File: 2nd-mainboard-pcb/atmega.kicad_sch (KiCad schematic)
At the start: 23 parts, among them J17 Fan_12/5V_Regelung, J2 Fan_12/5V_Regelung, J3 FAN0, J4 FAN1, J5 FAN2, J6 FAN3, U10 ATmega328PB-A, U7 TPM16050-S6TR, U8 RJK0456DPB-00-J5, U9 RJK0456DPB-00-J5, Y1 ECS-160-18-4X-CKM

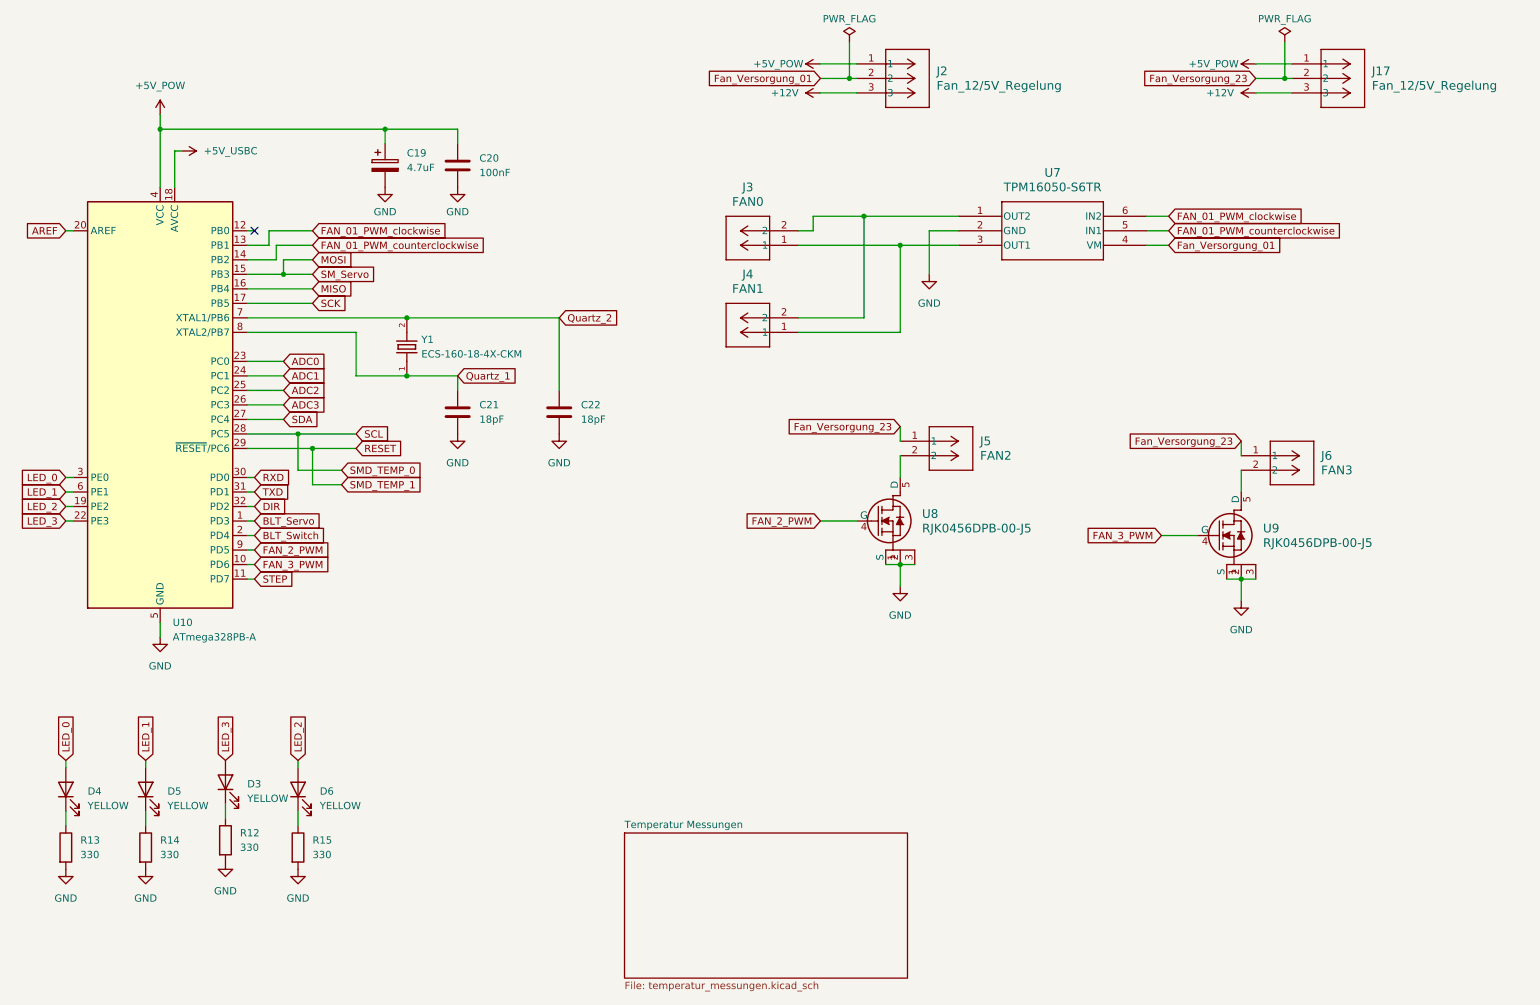
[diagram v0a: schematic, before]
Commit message: stacked pcb reworked
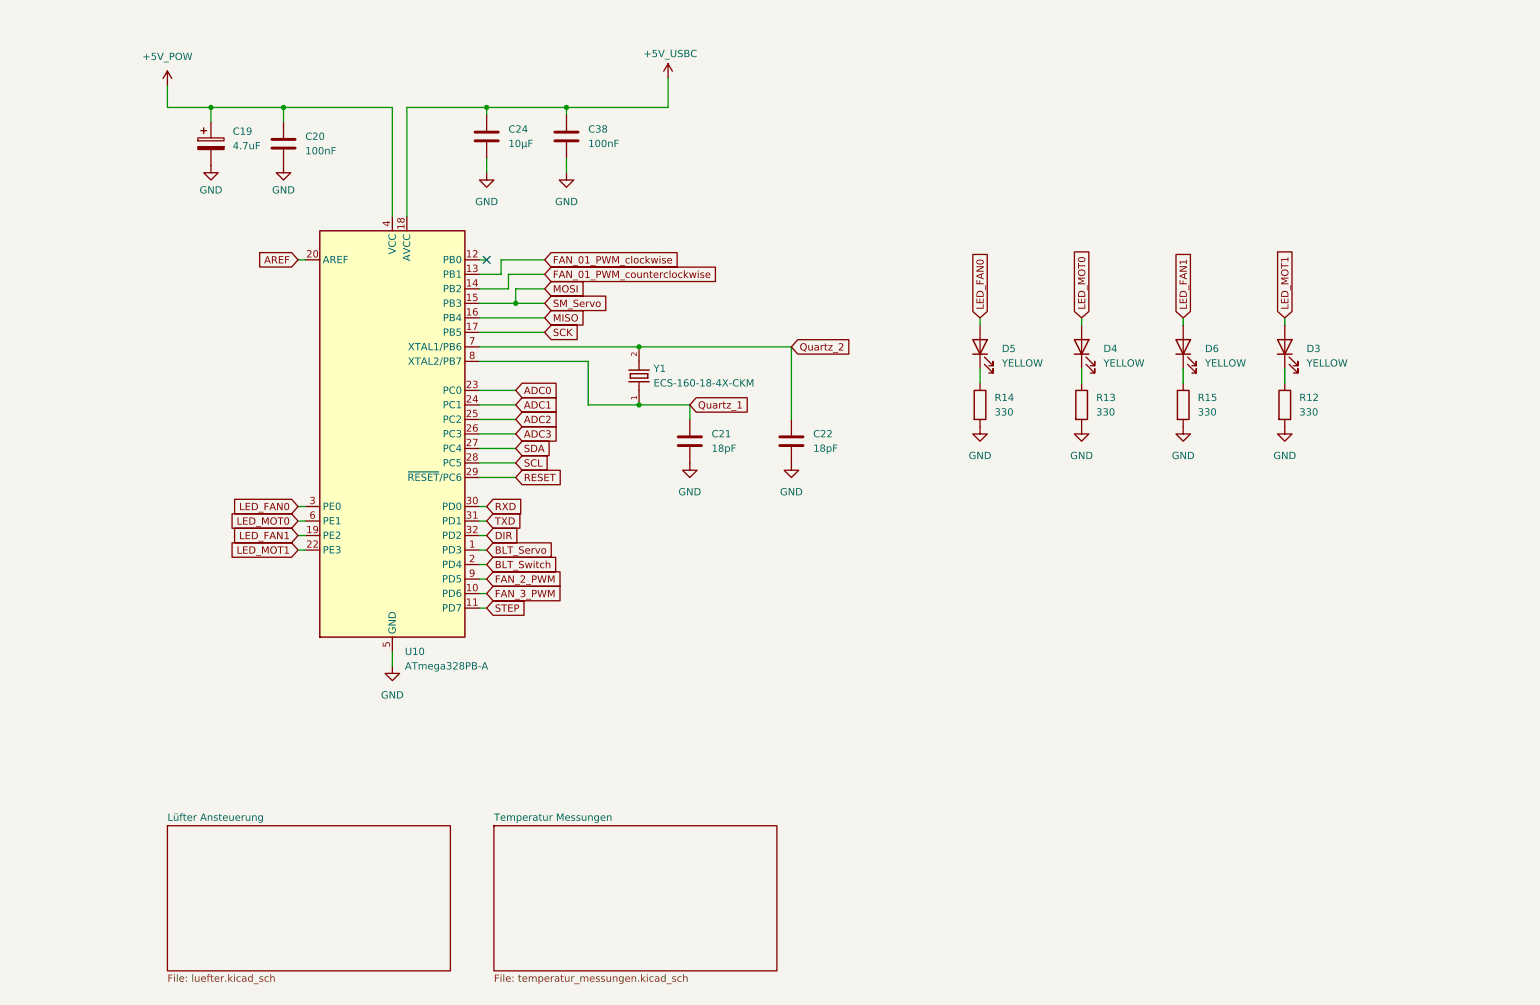
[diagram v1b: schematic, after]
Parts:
- removed J17, J2: Fan_12/5V_Regelung, Imported_Component_Footprints:FTS_103_01_F_S, symbol Imported_Component_Symbols:FTS-103-01-F-S
- removed J3: FAN0, Imported_Component_Footprints:CONN_S2B-XH-A-1LFSN_JST, symbol Imported_Component_Symbols:S2B-XH-A-1LFSN
- removed J4: FAN1, Imported_Component_Footprints:CONN_S2B-XH-A-1LFSN_JST, symbol Imported_Component_Symbols:S2B-XH-A-1LFSN
- removed J5: FAN2, Imported_Component_Footprints:CONN_S2B-XH-A-1LFSN_JST, symbol Imported_Component_Symbols:S2B-XH-A-1LFSN
- removed J6: FAN3, Imported_Component_Footprints:CONN_S2B-XH-A-1LFSN_JST, symbol Imported_Component_Symbols:S2B-XH-A-1LFSN
- removed U7: TPM16050-S6TR, Imported_Component_Footprints:TPM16050_S6TR, symbol Imported_Component_Symbols:TPM16050-S6TR
- removed U8, U9: RJK0456DPB-00-J5, Imported_Component_Footprints:RJK0456DPB_00_J5, symbol Imported_Component_Symbols:RJK0456DPB-00-J5
- added C24: 10µF, Capacitor_SMD:C_0805_2012Metric_Pad1.18x1.45mm_HandSolder, symbol Device:C
- added C38: 100nF, Capacitor_SMD:C_0402_1005Metric_Pad0.74x0.62mm_HandSolder, symbol Device:C
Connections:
- net +5V_USBC: now also C24.1, C38.1
- net GND: now also C24.2, C38.2
- net LED_0 renamed LED_FAN0
- net LED_FAN0: now also D5.2 (A); no longer D4.2 (A)
- net LED_1 renamed LED_MOT0
- net LED_MOT0: now also D4.2 (A); no longer D5.2 (A)
- net LED_2 renamed LED_FAN1
- net LED_3 renamed LED_MOT1
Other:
- added sheet Lüfter Ansteuerung (luefter.kicad_sch)
- moved on the sheet: C21, C22, D6, R15, U10, Y1

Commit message: rearragned componentens
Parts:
- C20, C21, C22, C38: footprint Capacitor_SMD:C_0402_1005Metric_Pad0.74x0.62mm_HandSolder -> Capacitor_SMD:C_0603_1608Metric_Pad1.08x0.95mm_HandSolder
- R12, R13, R14, R15: footprint Resistor_SMD:R_0402_1005Metric -> Resistor_SMD:R_0603_1608Metric_Pad0.98x0.95mm_HandSolder
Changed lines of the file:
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@@
 			)
 		)
-		(property "Footprint" "Resistor_SMD:R_0402_1005Metric"
+		(property "Footprint" "Resistor_SMD:R_0603_1608Metric_Pad0.98x0.95mm_HandSolder"
 			(at 178.562 88.9 90)
 			(effects
@@
 			)
 		)
-		(property "Footprint" "Resistor_SMD:R_0402_1005Metric"
+		(property "Footprint" "Resistor_SMD:R_0603_1608Metric_Pad0.98x0.95mm_HandSolder"
 			(at 214.122 88.9 90)
 			(effects
@@
 			)
 		)
-		(property "Footprint" "Resistor_SMD:R_0402_1005Metric"
+		(property "Footprint" "Resistor_SMD:R_0603_1608Metric_Pad0.98x0.95mm_HandSolder"
 			(at 231.902 88.9 90)
 			(effects
@@
 			)
 		)
-		(property "Footprint" "Capacitor_SMD:C_0402_1005Metric_Pad0.74x0.62mm_HandSolder"
+		(property "Footprint" "Capacitor_SMD:C_0603_1608Metric_Pad1.08x0.95mm_HandSolder"
 			(at 130.5052 99.06 0)
 			(effects
@@
 			)
 		)
-		(property "Footprint" "Capacitor_SMD:C_0402_1005Metric_Pad0.74x0.62mm_HandSolder"
+		(property "Footprint" "Capacitor_SMD:C_0603_1608Metric_Pad1.08x0.95mm_HandSolder"
 			(at 108.9152 45.72 0)
 			(effects
@@
 			)
 		)
-		(property "Footprint" "Resistor_SMD:R_0402_1005Metric"
+		(property "Footprint" "Resistor_SMD:R_0603_1608Metric_Pad0.98x0.95mm_HandSolder"
 			(at 196.342 88.9 90)
 			(effects
@@
 			)
 		)
-		(property "Footprint" "Capacitor_SMD:C_0402_1005Metric_Pad0.74x0.62mm_HandSolder"
+		(property "Footprint" "Capacitor_SMD:C_0603_1608Metric_Pad1.08x0.95mm_HandSolder"
 			(at 59.3852 46.99 0)
 			(effects
@@
 			)
 		)
-		(property "Footprint" "Capacitor_SMD:C_0402_1005Metric_Pad0.74x0.62mm_HandSolder"
+		(property "Footprint" "Capacitor_SMD:C_0603_1608Metric_Pad1.08x0.95mm_HandSolder"
 			(at 148.2852 99.06 0)
 			(effects
